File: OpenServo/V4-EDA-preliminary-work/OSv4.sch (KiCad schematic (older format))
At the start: 0 parts

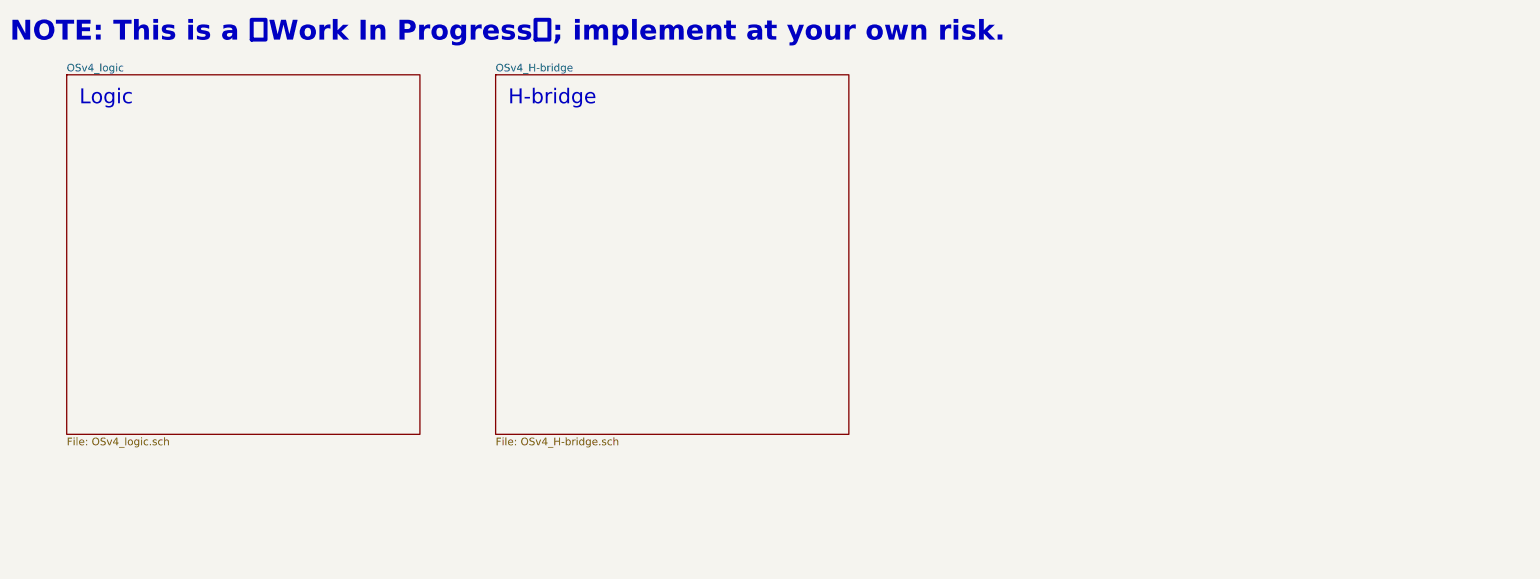
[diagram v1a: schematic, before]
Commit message: no message
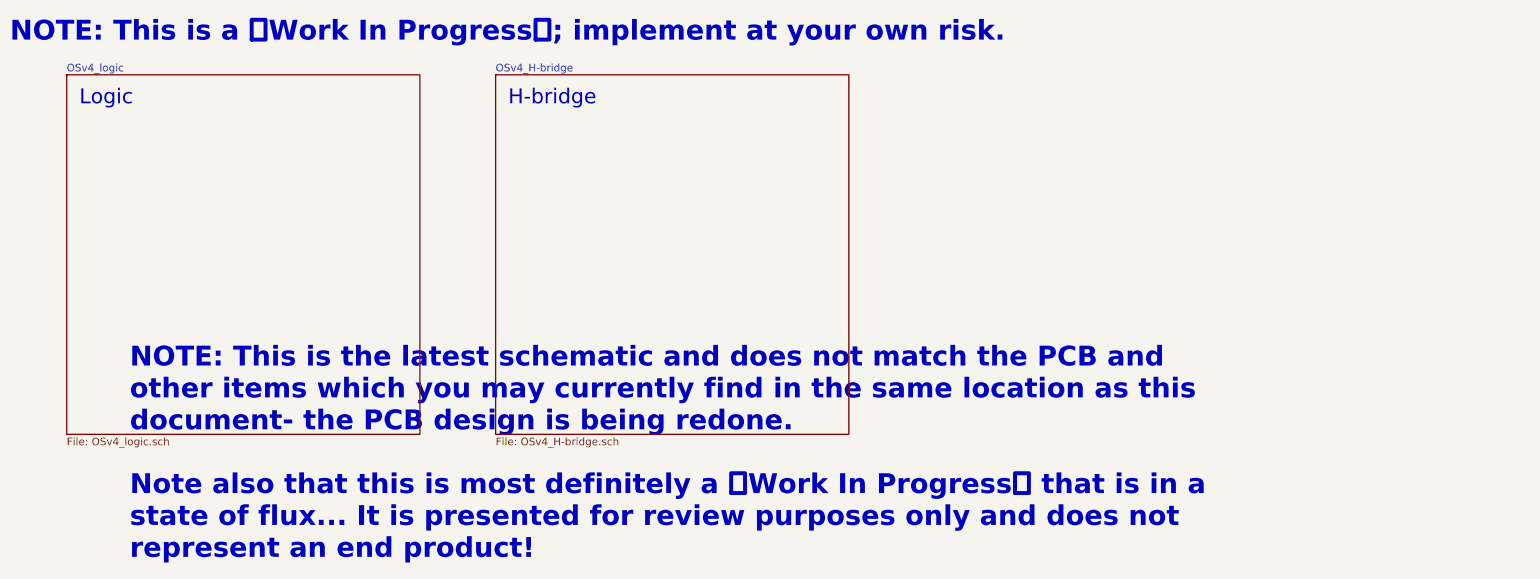
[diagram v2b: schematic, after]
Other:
- note added: "NOTE: This is the latest schematic and does not match the PCB and\nother items which you may currently find in the same location as this\ndocument- the PCB design is being redone.\n\nNote also that this is most definitely a Work In Progress that is in a\nstate of flux... It is presented for review purposes only and does not\nrepresent an end product!"
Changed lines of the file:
@@
-EESchema Schematic File Version 2  date 04/05/2010 11:09:49
+EESchema Schematic File Version 2  date 07/05/2010 17:07:47
 LIBS:power
 LIBS:device
@@
 Sheet 1 3
 Title "OpenServo v4 preliminary work-up, © OpenServo project 2010"
-Date "4 may 2010"
+Date "7 may 2010"
 Rev ""
 Comp ""
@@
 Comment4 ""
 $EndDescr
+Text Notes 1550 4900 0    157  ~ 31
+NOTE: This is the latest schematic and does not match the PCB and\nother items which you may currently find in the same location as this\ndocument- the PCB design is being redone.\n\nNote also that this is most definitely a Work In Progress that is in a\nstate of flux... It is presented for review purposes only and does not\nrepresent an end product!
 Text Notes 600  800  0    157  ~ 31
 NOTE: This is a Work In Progress; implement at your own risk.
